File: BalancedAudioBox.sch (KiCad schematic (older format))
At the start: 5 parts, among them J1 Conn_02x10_Odd_Even, J2 Conn_01x03, J5 Conn_01x03, J7 Conn_01x05

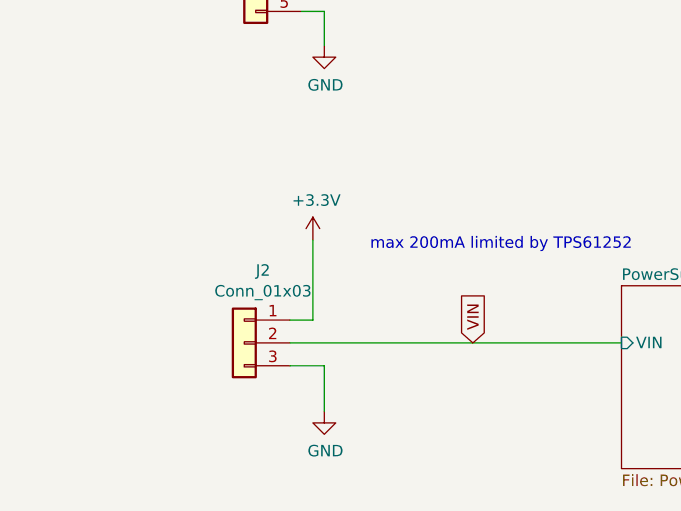
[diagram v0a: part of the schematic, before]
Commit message: more layout
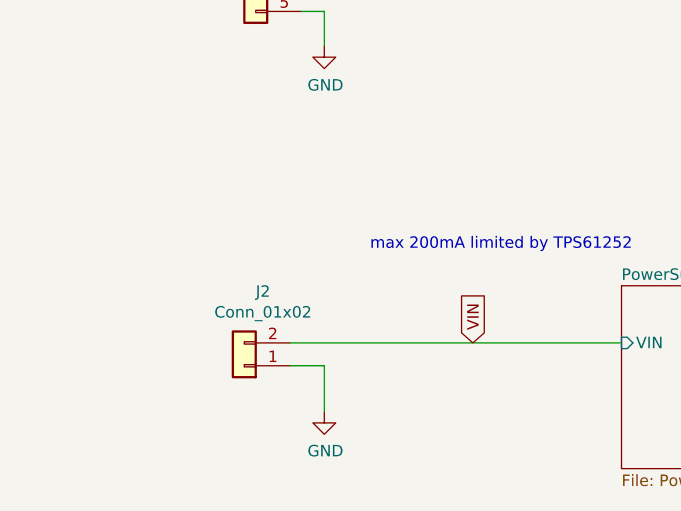
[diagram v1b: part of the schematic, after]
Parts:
- removed J2: Conn_01x03, Connector_PinHeader_2.54mm:PinHeader_1x03_P2.54mm_Vertical, symbol Connector_Generic:Conn_01x03
- added J2: Conn_01x02, Connector_PinHeader_2.54mm:PinHeader_1x02_P2.54mm_Vertical, symbol Connector_Generic:Conn_01x02
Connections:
- net GND: now also J2.1 (Pin_1)
- net VIN: now also J2.2 (Pin_2)
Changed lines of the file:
@@
 NoConn ~ 3450 2300
-$Comp
-L Connector_Generic:Conn_01x03 J2
-U 1 1 5D436D81
-P 2950 5950
-F 0 "J2" H 2868 6267 50  0000 C CNN
-F 1 "Conn_01x03" H 2868 6176 50  0000 C CNN
-F 2 "Connector_PinHeader_2.54mm:PinHeader_1x03_P2.54mm_Vertical" H 2950 5950 50  0001 C CNN
-F 3 "~" H 2950 5950 50  0001 C CNN
-	1    2950 5950
-	-1   0    0    -1
-$EndComp
-$Comp
-L power:+3.3V #PWR0101
-U 1 1 5D437E68
-P 3250 5500
-F 0 "#PWR0101" H 3250 5350 50  0001 C CNN
-F 1 "+3.3V" H 3265 5673 50  0000 C CNN
-F 2 "" H 3250 5500 50  0001 C CNN
-F 3 "" H 3250 5500 50  0001 C CNN
-	1    3250 5500
-	1    0    0    -1
-$EndComp
-Wire Wire Line
-	3150 5850 3250 5850
-Wire Wire Line
-	3250 5850 3250 5500
 $Comp
 L Connector_Generic:Conn_01x03 J5
@@
 Text GLabel 3950 5950 1    50   Input ~ 0
 VIN
+$Comp
+L Connector_Generic:Conn_01x02 J2
+U 1 1 5D4B761F
+P 2950 6050
+F 0 "J2" H 2868 5725 50  0000 C CNN
+F 1 "Conn_01x02" H 2868 5816 50  0000 C CNN
+F 2 "Connector_PinHeader_2.54mm:PinHeader_1x02_P2.54mm_Vertical" H 2950 6050 50  0001 C CNN
+F 3 "~" H 2950 6050 50  0001 C CNN
+	1    2950 6050
+	-1   0    0    1
+$EndComp
 $EndSCHEMATC
